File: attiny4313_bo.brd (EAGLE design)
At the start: 49.5 x 22.2 mm, 11 parts, among them J1 AVR_SPI_PRG_6NS, Y1 16MHz

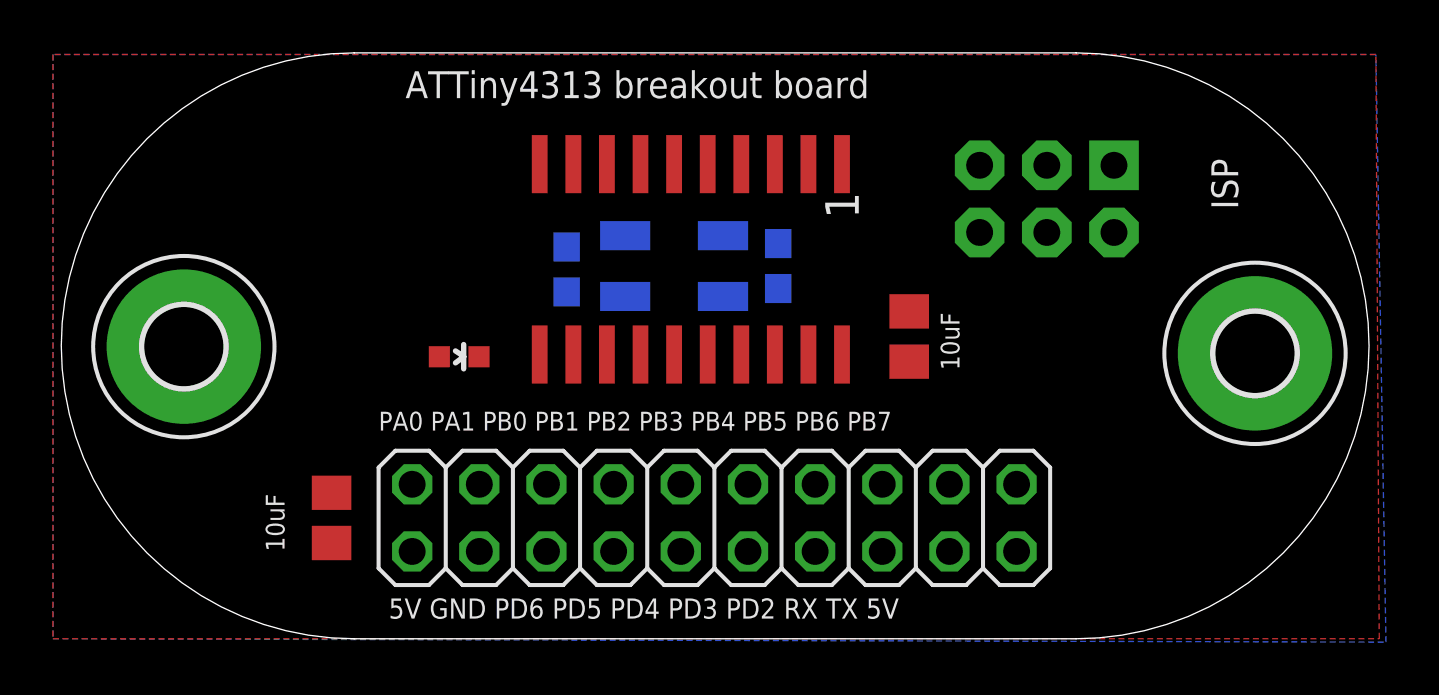
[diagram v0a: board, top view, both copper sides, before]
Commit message: routed
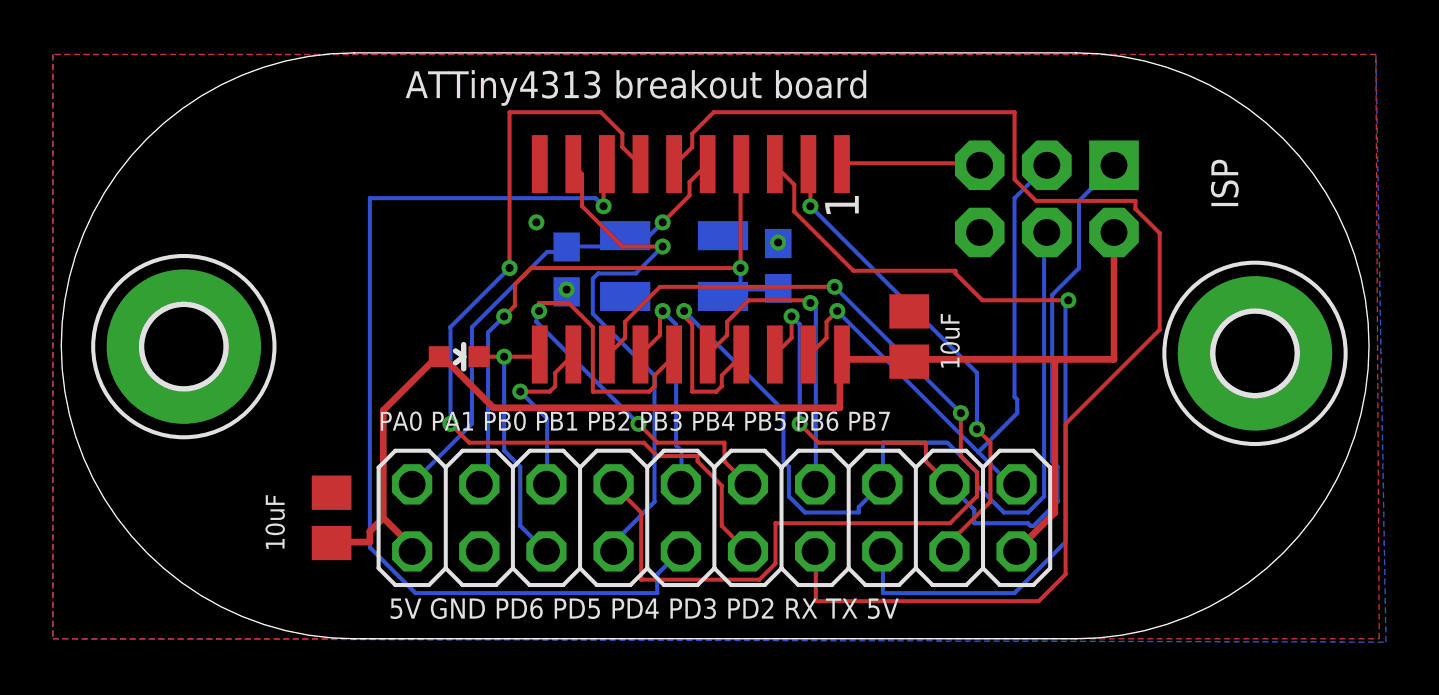
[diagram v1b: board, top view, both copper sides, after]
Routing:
- net +5V: track 0.00 -> 52.6 mm
- net PD2: track 0.00 -> 49.2 mm
- net PB1: track 0.00 -> 39.1 mm, vias 0 -> 2
- net PB5/MOSI: track 0.00 -> 38.2 mm, vias 0 -> 1
- net PD4: track 0.00 -> 37.4 mm, vias 0 -> 1
- net PD3: track 0.00 -> 33.0 mm, vias 0 -> 2
- net PD1/TXD: track 0.00 -> 32.4 mm, vias 0 -> 1
- net PB6/MISO: track 0.00 -> 32.1 mm, vias 0 -> 2
- net PA1/XTAL2: track 0.00 -> 24.7 mm, vias 0 -> 2
- net PB7/SCL: track 0.00 -> 23.6 mm, vias 0 -> 1
- net PB3: track 0.00 -> 20.5 mm, vias 0 -> 2
- net PD5: track 0.00 -> 20.5 mm, vias 0 -> 1
- net PA0/XTAL1: track 0.00 -> 19.0 mm, vias 0 -> 1
- net PD0/RDX: track 0.00 -> 18.1 mm, vias 0 -> 2
- net PB4: track 0.00 -> 12.1 mm, vias 0 -> 1
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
